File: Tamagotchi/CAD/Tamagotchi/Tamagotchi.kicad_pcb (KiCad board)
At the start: 2 copper layers, 19 parts, among them J1 Conn_01x06_Pin, SW1 SW_Push, SW2 SW_Push, SW3 SW_Push, SW4 SW_Push, SW5 SW_SPDT, U1 ESP32-C3-SuperMini, U2 SSD1306

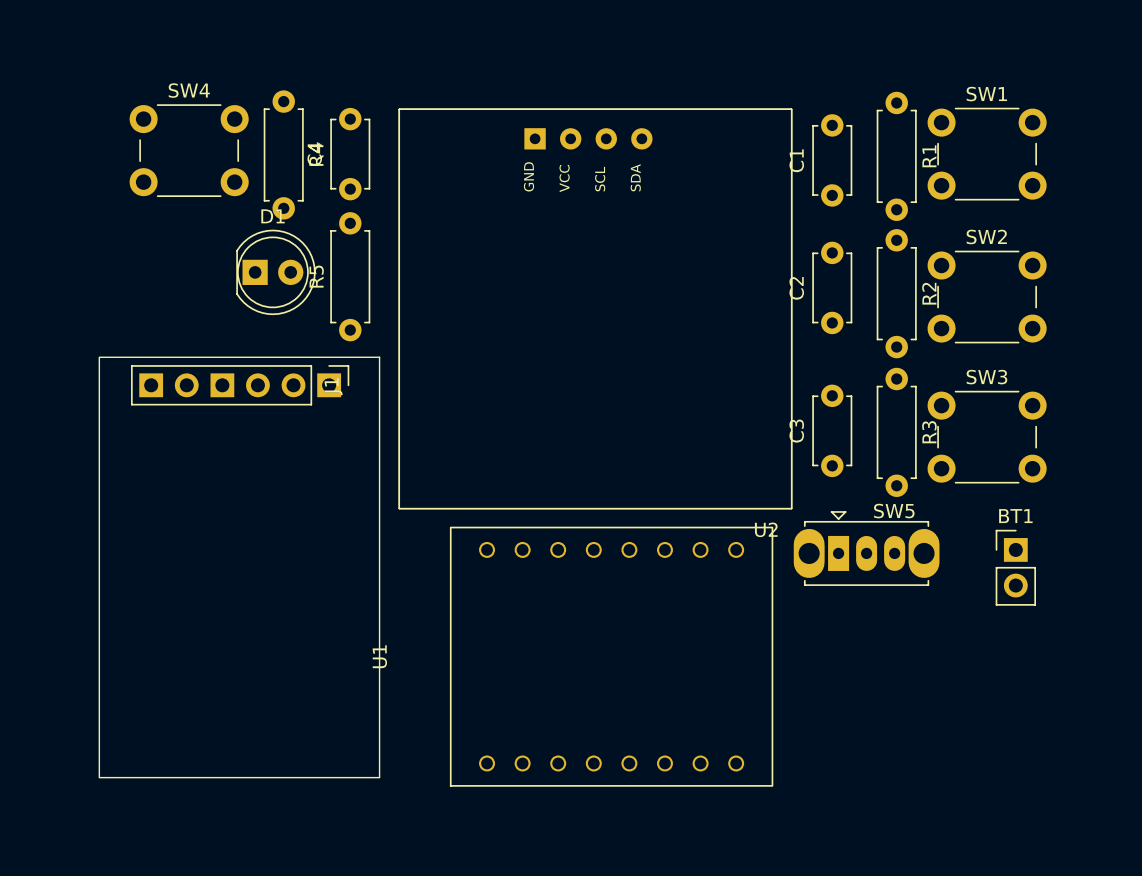
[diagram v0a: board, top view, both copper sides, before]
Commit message: updated Tamagotchi
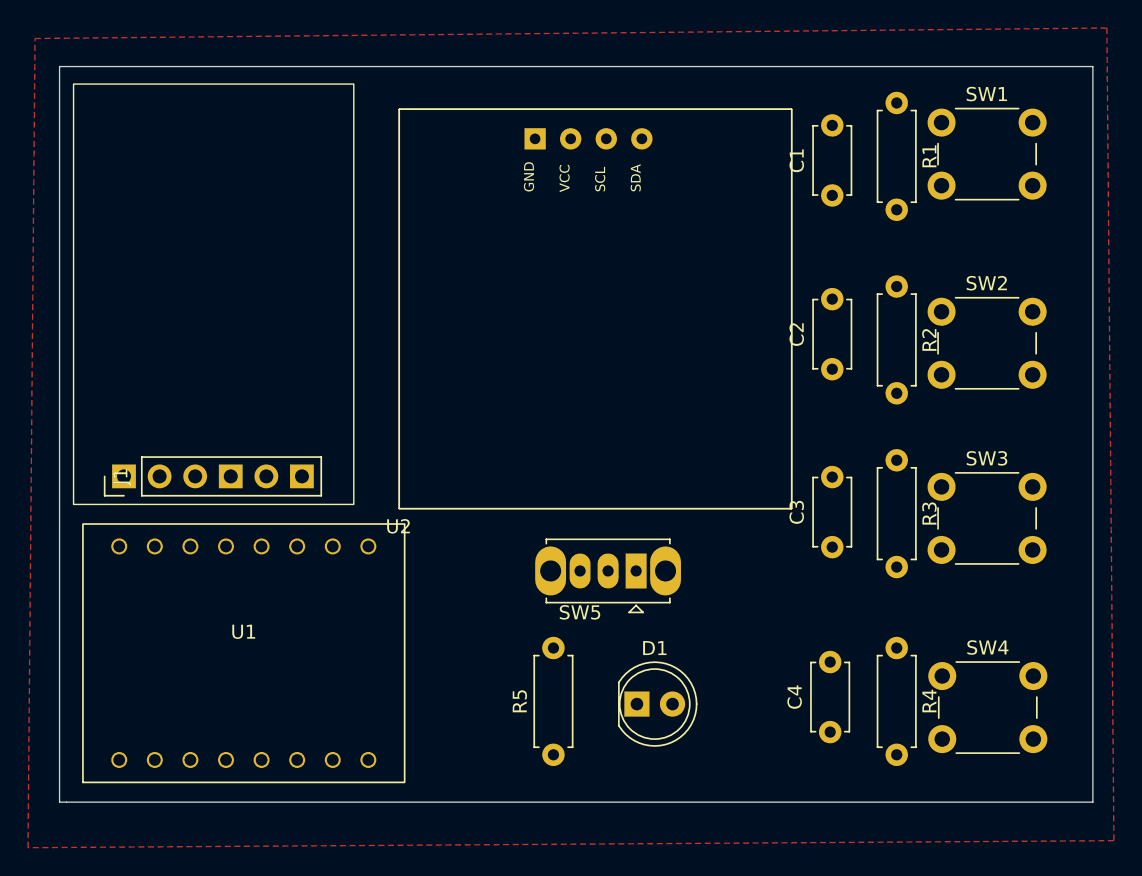
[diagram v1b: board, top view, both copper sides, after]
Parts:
- removed BT1: Battery_Cell, Connector_PinHeader_2.54mm:PinHeader_1x02_P2.54mm_Vertical
- moved SW4 69.5 mm to (160.2, 106.0)
- moved R4 58.6 mm to (157.0, 104.0)
- moved C4 51.7 mm to (152.2, 110.0)
- moved D1 41.1 mm to (138.5, 108.0)
- moved R5 33.6 mm to (132.5, 111.6)
- moved U1 26.3 mm to (110.4, 104.4)
- moved J1 15.3 mm to (102.2, 91.8), turned to 90 degrees
- moved SW5 14.5 mm to (138.4, 98.5), turned to 180 degrees
- moved C3 5.80 mm to (152.4, 96.8)
- moved R3 5.80 mm to (157.0, 90.6)
- moved SW3 5.80 mm to (160.2, 92.5)
- moved C2 3.30 mm to (152.4, 84.1)
- moved R2 3.30 mm to (157.0, 78.2)
- moved SW2 3.30 mm to (160.2, 80.0)
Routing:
- added copper zone on F.Cu, net (none)
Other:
- board outline added: 73.8 x 52.5 mm
